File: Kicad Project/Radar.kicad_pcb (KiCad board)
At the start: 2 copper layers, 104.1 x 101.6 mm, 46 parts, among them U1 GALI-1+, U10 GALI-2+, U2 MCA1-85L+, U4 LMV751, U5 LMV751, U6 GALI-2+, U7 RMK-3-93+, U8 GALI-2+, U9 LEE-39+

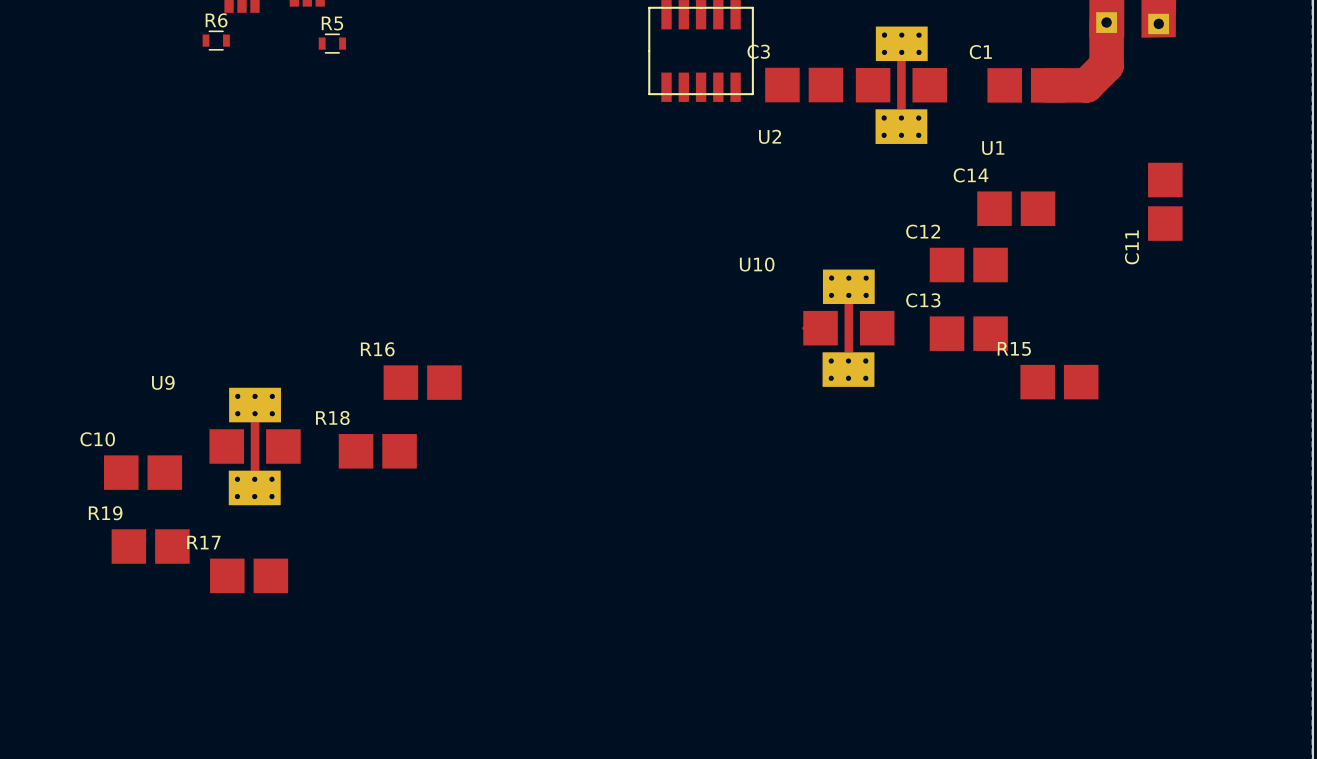
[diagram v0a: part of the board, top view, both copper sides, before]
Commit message: asdf
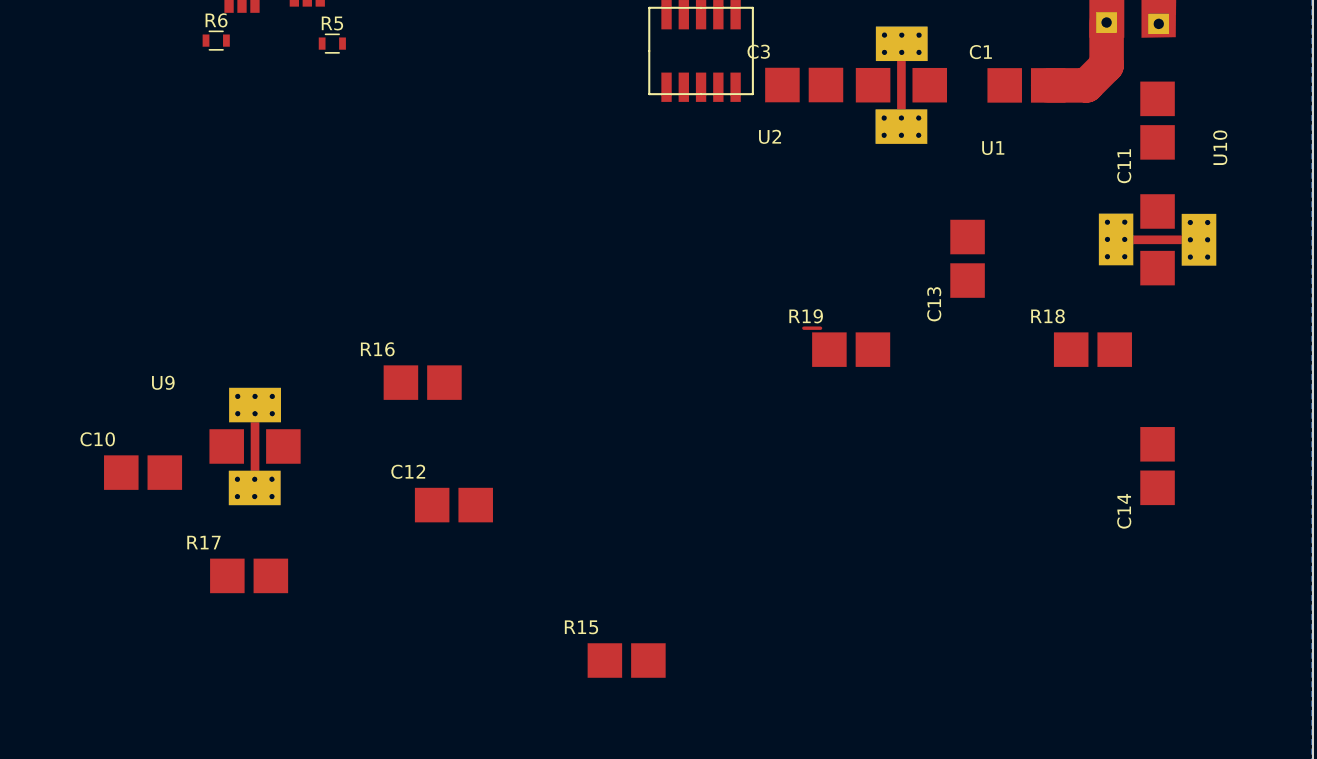
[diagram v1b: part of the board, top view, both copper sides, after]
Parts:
- moved R19 53.5 mm to (163.8, 143.5)
- moved R18 53.1 mm to (181.6, 143.5)
- moved C12 41.8 mm to (134.6, 154.9)
- moved R15 37.8 mm to (147.3, 166.4)
- moved U10 23.8 mm to (185.4, 133.3), turned to 270 degrees
- moved C14 21.6 mm to (188.0, 151.1), turned to 90 degrees
- moved C13 6.62 mm to (174.0, 135.9), turned to 90 degrees
- moved C11 6.00 mm to (188.0, 125.7)
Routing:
- net Net-(C11-Pad1): track 1.23 -> 0.00 mm
- net (no net): track 0.00 -> 1.23 mm
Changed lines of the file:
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@@
     (links 136)
     (no_connects 52)
-    (area 93.904999 76.124999 198.195001 177.875001)
+    (area 93.904999 64.6811 228.422201 177.875001)
     (thickness 1.6)
     (drawings 48)
@@
   )
   (setup
-    (last_trace_width 2.54)
+    (last_trace_width 0.25)
     (user_trace_width 0.254)
     (user_trace_width 0.508)
@@
   )
   (module RadarComponents:Amplifier (layer F.Cu)
-    (at 163.17799 141.9332)
-    (fp_text reference U10 (at -5.9436 -5.9182) (layer F.SilkS)
-      (effects (font (size 1 1) (thickness 0.15)))
-    )
-    (fp_text value GALI-2+ (at 4.1656 -6.1468) (layer F.Fab)
-      (effects (font (size 1 1) (thickness 0.15)))
-    )
-    (pad 2 thru_hole rect (at 0.7874 2.413) (size 1.27 1.27) (drill 0.381) (layers *.Cu *.Mask)
-      (net 9 GND))
-    (pad 2 thru_hole rect (at 2.0574 2.413) (size 1.27 1.27) (drill 0.381) (layers *.Cu *.Mask)
-      (net 9 GND))
-    (pad 2 thru_hole rect (at -0.4826 2.413) (size 1.27 1.27) (drill 0.381) (layers *.Cu *.Mask)
-      (net 9 GND))
-    (pad 2 thru_hole rect (at -0.4826 1.143) (size 1.27 1.27) (drill 0.381) (layers *.Cu *.Mask)
-      (net 9 GND))
-    (pad 2 thru_hole rect (at 0.7874 1.143) (size 1.27 1.27) (drill 0.381) (layers *.Cu *.Mask)
-      (net 9 GND))
-    (pad 2 thru_hole rect (at 2.0574 1.143) (size 1.27 1.27) (drill 0.381) (layers *.Cu *.Mask)
-      (net 9 GND))
-    (pad 2 thru_hole rect (at 2.0828 -4.953) (size 1.27 1.27) (drill 0.381) (layers *.Cu *.Mask)
-      (net 9 GND))
-    (pad 2 thru_hole rect (at 0.8128 -4.953) (size 1.27 1.27) (drill 0.381) (layers *.Cu *.Mask)
-      (net 9 GND))
-    (pad 2 thru_hole rect (at -0.4572 -4.953) (size 1.27 1.27) (drill 0.381) (layers *.Cu *.Mask)
-      (net 9 GND))
-    (pad 2 thru_hole rect (at -0.4572 -3.683) (size 1.27 1.27) (drill 0.381) (layers *.Cu *.Mask)
-      (net 9 GND))
-    (pad 2 thru_hole rect (at 2.0828 -3.683) (size 1.27 1.27) (drill 0.381) (layers *.Cu *.Mask)
-      (net 9 GND))
-    (pad 3 smd rect (at 2.8956 -1.27) (size 2.54 2.54) (layers F.Cu F.Paste F.Mask)
+    (at 185.42 133.35 270)
+    (fp_text reference U10 (at -5.9436 -5.9182 270) (layer F.SilkS)
+      (effects (font (size 1 1) (thickness 0.15)))
+    )
+    (fp_text value GALI-2+ (at 4.1656 -6.1468 270) (layer F.Fab)
+      (effects (font (size 1 1) (thickness 0.15)))
+    )
+    (pad 2 thru_hole rect (at 0.7874 2.413 270) (size 1.27 1.27) (drill 0.381) (layers *.Cu *.Mask)
+      (net 9 GND))
+    (pad 2 thru_hole rect (at 2.0574 2.413 270) (size 1.27 1.27) (drill 0.381) (layers *.Cu *.Mask)
+      (net 9 GND))
+    (pad 2 thru_hole rect (at -0.4826 2.413 270) (size 1.27 1.27) (drill 0.381) (layers *.Cu *.Mask)
+      (net 9 GND))
+    (pad 2 thru_hole rect (at -0.4826 1.143 270) (size 1.27 1.27) (drill 0.381) (layers *.Cu *.Mask)
+      (net 9 GND))
+    (pad 2 thru_hole rect (at 0.7874 1.143 270) (size 1.27 1.27) (drill 0.381) (layers *.Cu *.Mask)
+      (net 9 GND))
+    (pad 2 thru_hole rect (at 2.0574 1.143 270) (size 1.27 1.27) (drill 0.381) (layers *.Cu *.Mask)
+      (net 9 GND))
+    (pad 2 thru_hole rect (at 2.0828 -4.953 270) (size 1.27 1.27) (drill 0.381) (layers *.Cu *.Mask)
+      (net 9 GND))
+    (pad 2 thru_hole rect (at 0.8128 -4.953 270) (size 1.27 1.27) (drill 0.381) (layers *.Cu *.Mask)
+      (net 9 GND))
+    (pad 2 thru_hole rect (at -0.4572 -4.953 270) (size 1.27 1.27) (drill 0.381) (layers *.Cu *.Mask)
+      (net 9 GND))
+    (pad 2 thru_hole rect (at -0.4572 -3.683 270) (size 1.27 1.27) (drill 0.381) (layers *.Cu *.Mask)
+      (net 9 GND))
+    (pad 2 thru_hole rect (at 2.0828 -3.683 270) (size 1.27 1.27) (drill 0.381) (layers *.Cu *.Mask)
+      (net 9 GND))
+    (pad 3 smd rect (at 2.8956 -1.27 270) (size 2.54 2.54) (layers F.Cu F.Paste F.Mask)
       (net 28 "Net-(C14-Pad2)"))
-    (pad 1 smd rect (at -1.27 -1.27) (size 2.54 2.54) (layers F.Cu F.Paste F.Mask)
+    (pad 1 smd rect (at -1.27 -1.27 270) (size 2.54 2.54) (layers F.Cu F.Paste F.Mask)
       (net 17 "Net-(C11-Pad1)"))
-    (pad 2 smd rect (at 0.8128 -1.27) (size 0.635 3.556) (layers F.Cu F.Paste F.Mask)
-      (net 9 GND))
-    (pad 2 thru_hole rect (at 0.8128 -3.683) (size 1.27 1.27) (drill 0.381) (layers *.Cu *.Mask)
+    (pad 2 smd rect (at 0.8128 -1.27 270) (size 0.635 3.556) (layers F.Cu F.Paste F.Mask)
+      (net 9 GND))
+    (pad 2 thru_hole rect (at 0.8128 -3.683 270) (size 1.27 1.27) (drill 0.381) (layers *.Cu *.Mask)
       (net 9 GND))
   )
@@
   )
   (module RadarComponents:100PAD (layer F.Cu)
-    (at 188.5315 131.699 90)
+    (at 187.96 125.73 90)
     (fp_text reference C11 (at -2.9972 -3.683 90) (layer F.SilkS)
       (effects (font (size 1 1) (thickness 0.15)))
@@
   )
   (module RadarComponents:100PAD (layer F.Cu)
-    (at 172.480581 137.2864)
+    (at 134.62 154.94)
     (fp_text reference C12 (at -2.9972 -3.683) (layer F.SilkS)
       (effects (font (size 1 1) (thickness 0.15)))
@@
   )
   (module RadarComponents:100PAD (layer F.Cu)
-    (at 172.480581 142.3364)
-    (fp_text reference C13 (at -2.9972 -3.683) (layer F.SilkS)
-      (effects (font (size 1 1) (thickness 0.15)))
-    )
-    (fp_text value 150p (at 5.842 -3.683) (layer F.Fab)
-      (effects (font (size 1 1) (thickness 0.15)))
-    )
-    (pad 2 smd rect (at 1.9304 -1.27) (size 2.54 2.54) (layers F.Cu F.Paste F.Mask)
-      (net 9 GND))
-    (pad 1 smd rect (at -1.27 -1.27) (size 2.54 2.54) (layers F.Cu F.Paste F.Mask)
+    (at 173.99 135.89 90)
+    (fp_text reference C13 (at -2.9972 -3.683 90) (layer F.SilkS)
+      (effects (font (size 1 1) (thickness 0.15)))
+    )
+    (fp_text value 150p (at 5.842 -3.683 90) (layer F.Fab)
+      (effects (font (size 1 1) (thickness 0.15)))
+    )
+    (pad 2 smd rect (at 1.9304 -1.27 90) (size 2.54 2.54) (layers F.Cu F.Paste F.Mask)
+      (net 9 GND))
+    (pad 1 smd rect (at -1.27 -1.27 90) (size 2.54 2.54) (layers F.Cu F.Paste F.Mask)
       (net 27 "Net-(C13-Pad1)"))
   )
   (module RadarComponents:100PAD (layer F.Cu)
-    (at 175.9712 133.1468)
-    (fp_text reference C14 (at -2.9972 -3.683) (layer F.SilkS)
-      (effects (font (size 1 1) (thickness 0.15)))
-    )
-    (fp_text value 150p (at 5.842 -3.683) (layer F.Fab)
-      (effects (font (size 1 1) (thickness 0.15)))
-    )
-    (pad 2 smd rect (at 1.9304 -1.27) (size 2.54 2.54) (layers F.Cu F.Paste F.Mask)
+    (at 187.96 151.13 90)
+    (fp_text reference C14 (at -2.9972 -3.683 90) (layer F.SilkS)
+      (effects (font (size 1 1) (thickness 0.15)))
+    )
+    (fp_text value 150p (at 5.842 -3.683 90) (layer F.Fab)
+      (effects (font (size 1 1) (thickness 0.15)))
+    )
+    (pad 2 smd rect (at 1.9304 -1.27 90) (size 2.54 2.54) (layers F.Cu F.Paste F.Mask)
       (net 28 "Net-(C14-Pad2)"))
-    (pad 1 smd rect (at -1.27 -1.27) (size 2.54 2.54) (layers F.Cu F.Paste F.Mask)
+    (pad 1 smd rect (at -1.27 -1.27 90) (size 2.54 2.54) (layers F.Cu F.Paste F.Mask)
       (net 29 "Net-(C14-Pad1)"))
   )
@@
   )
   (module RadarComponents:100PAD (layer F.Cu)
-    (at 179.1462 145.8976)
+    (at 147.32 166.37)
     (fp_text reference R15 (at -2.9972 -3.683) (layer F.SilkS)
       (effects (font (size 1 1) (thickness 0.15)))
@@
   )
   (module RadarComponents:100PAD (layer F.Cu)
-    (at 129.021981 150.985)
+    (at 181.61 143.51)
     (fp_text reference R18 (at -2.9972 -3.683) (layer F.SilkS)
       (effects (font (size 1 1) (thickness 0.15)))
@@
   )
   (module RadarComponents:100PAD (layer F.Cu)
-    (at 112.3188 157.988)
+    (at 163.83 143.51)
     (fp_text reference R19 (at -2.9972 -3.683) (layer F.SilkS)
       (effects (font (size 1 1) (thickness 0.15)))
@@
   (gr_line (start 93.98 76.2) (end 198.12 76.2) (angle 90) (layer Edge.Cuts) (width 0.15))
   (gr_line (start 93.98 177.8) (end 93.98 76.2) (angle 90) (layer Edge.Cuts) (width 0.15))
+  (segment (start 161.90799 140.6632) (end 160.6824 140.6632) (width 0.25) (layer F.Cu) (net 0))
   (segment (start 108.458 94.869) (end 104.4702 94.869) (width 2.54) (layer F.Cu) (net 1))
   (segment (start 104.2416 94.6404) (end 104.2416 94.2848) (width 2.54) (layer F.Cu) (net 1))
@@
   (segment (start 121.031 105.0036) (end 121.0437 105.0163) (width 2.54) (layer F.Cu) (net 14))
   (segment (start 170.2181 104.0384) (end 170.2181 110.0201) (width 2.54) (layer F.Cu) (net 15))
-  (segment (start 161.90799 140.6632) (end 160.6824 140.6632) (width 0.25) (layer F.Cu) (net 17))
   (segment (start 133.985 94.869) (end 133.985 91.8972) (width 2.54) (layer F.Cu) (net 24))
   (segment (start 133.985 94.869) (end 131.0386 94.869) (width 2.54) (layer F.Cu) (net 24))
   (segment (start 140.335 94.869) (end 137.1854 94.869) (width 2.54) (layer F.Cu) (net 25))
-  (segment (start 182.9435 118.1862) (end 182.9435 121.3358) (width 2.54) (layer F.Cu) (net 35) (status 400000))
-  (segment (start 181.4703 122.809) (end 178.6509 122.809) (width 2.54) (layer F.Cu) (net 35) (status 800000))
+  (segment (start 182.9435 118.1862) (end 182.9435 121.3358) (width 2.54) (layer F.Cu) (net 35))
+  (segment (start 181.4703 122.809) (end 178.6509 122.809) (width 2.54) (layer F.Cu) (net 35))
   (segment (start 182.9435 121.3358) (end 181.4703 122.809) (width 2.54) (layer F.Cu) (net 35))
   (segment (start 134.0358 85.5472) (end 134.0358 88.646) (width 2.54) (layer F.Cu) (net 37) (status 20))
-  (segment (start 176.3776 100.838) (end 183.7055 100.838) (width 2.54) (layer F.Cu) (net 39) (status 400000))
-  (segment (start 184.8231 101.9556) (end 184.8231 104.5718) (width 2.54) (layer F.Cu) (net 39) (status 800000))
+  (segment (start 176.3776 100.838) (end 183.7055 100.838) (width 2.54) (layer F.Cu) (net 39))
+  (segment (start 184.8231 101.9556) (end 184.8231 104.5718) (width 2.54) (layer F.Cu) (net 39))
   (segment (start 183.7055 100.838) (end 184.8231 101.9556) (width 2.54) (layer F.Cu) (net 39))
   (zone (net 9) (net_name GND) (layer B.Cu) (hatch edge 0.508)
